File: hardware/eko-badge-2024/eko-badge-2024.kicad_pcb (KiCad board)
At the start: 2 copper layers, 47.5 x 108.1 mm, 56 parts, among them J1 UART, J2 Battery, J3 Lentes, J4 OLED, J5 Add-On, J6 Add-On, J7 Battery, P1 USB_C_Plug_USB2.0, Q1 DMG3415U-7, SW1 ON, SW2 LEFT, SW3 UP, SW4 DOWN, SW5 RESET, SW6 BOOT, SW7 RIGTH, U1 ESP32-C6-WROOM-1-N4, U2 XC6220B331MR-G, U3 RFM95W-868S2, U4 TPA321

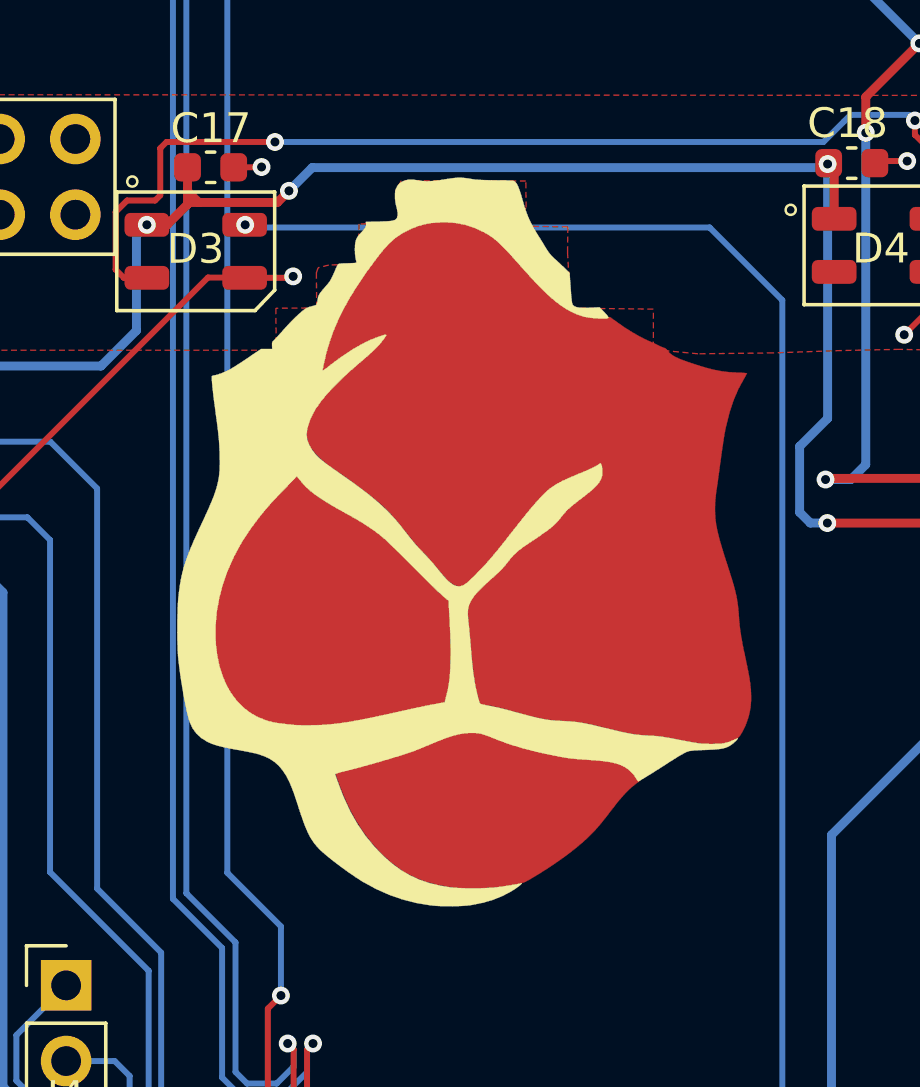
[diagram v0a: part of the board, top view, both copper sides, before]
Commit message: feeat(Hw):Added_New_Cut
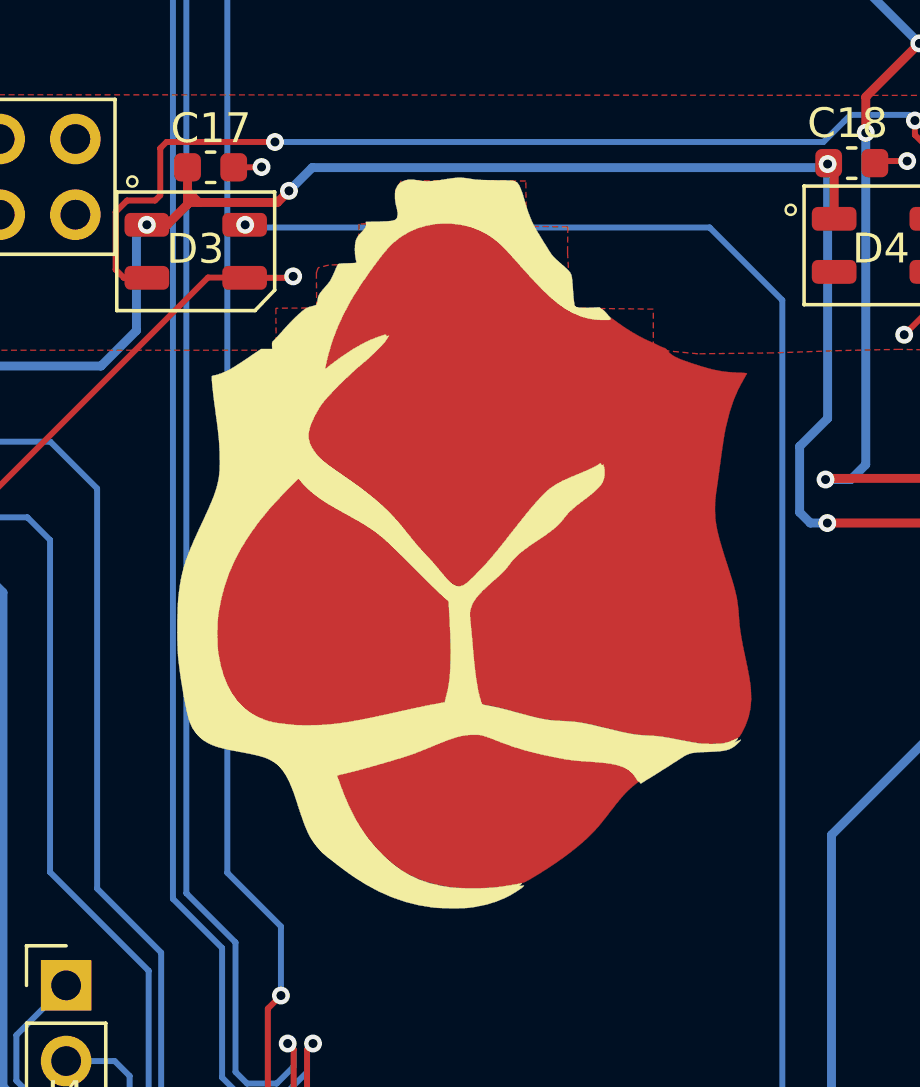
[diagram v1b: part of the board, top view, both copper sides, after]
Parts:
- moved Ref** 0.29 mm to (203.7, 84.0)
